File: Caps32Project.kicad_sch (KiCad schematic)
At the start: 37 parts, among them J1 Ph 2.0, J2 Sh 1.0, J4 Sh 2.0, P1 USB_C_Plug_USB2.0, Q1 AO3401A, Q2 MBT3904DW1, SW1 Reset, SW2 Boot, U1 MPU-6050, U2 MAX17048G_T10, U4 MCP73831-2-OT, U5 AP2112K-3.3, U6 ESP32-WROOM-32D

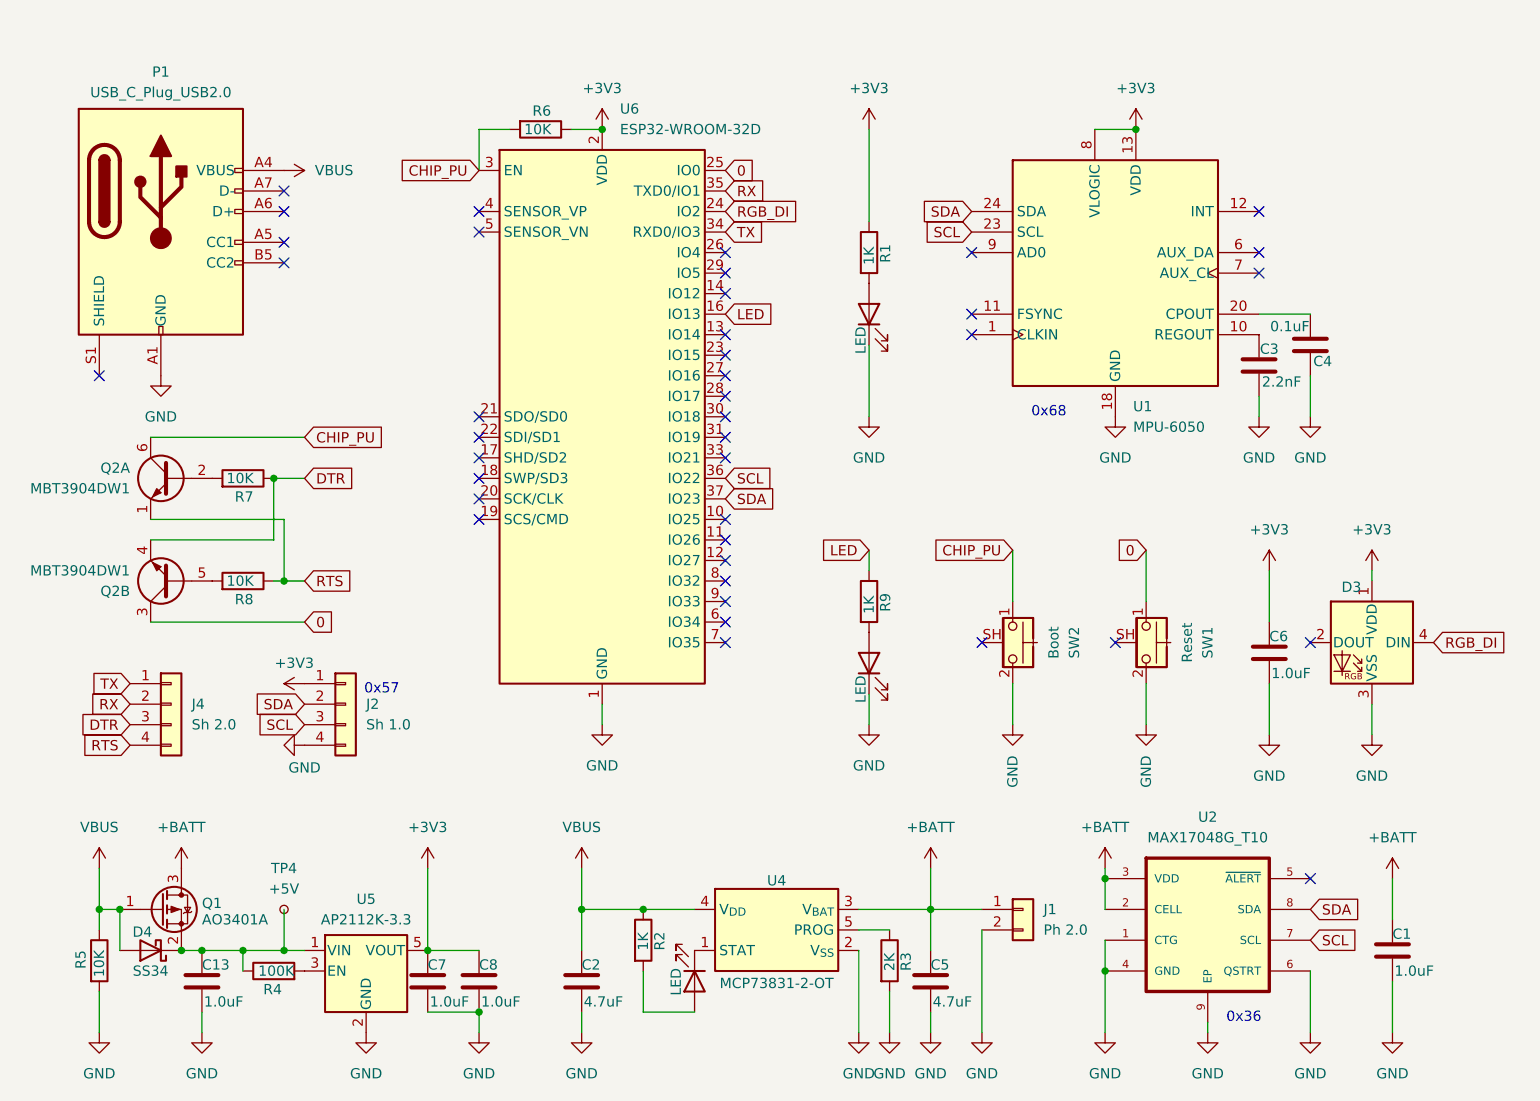
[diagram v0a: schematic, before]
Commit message: Update Board
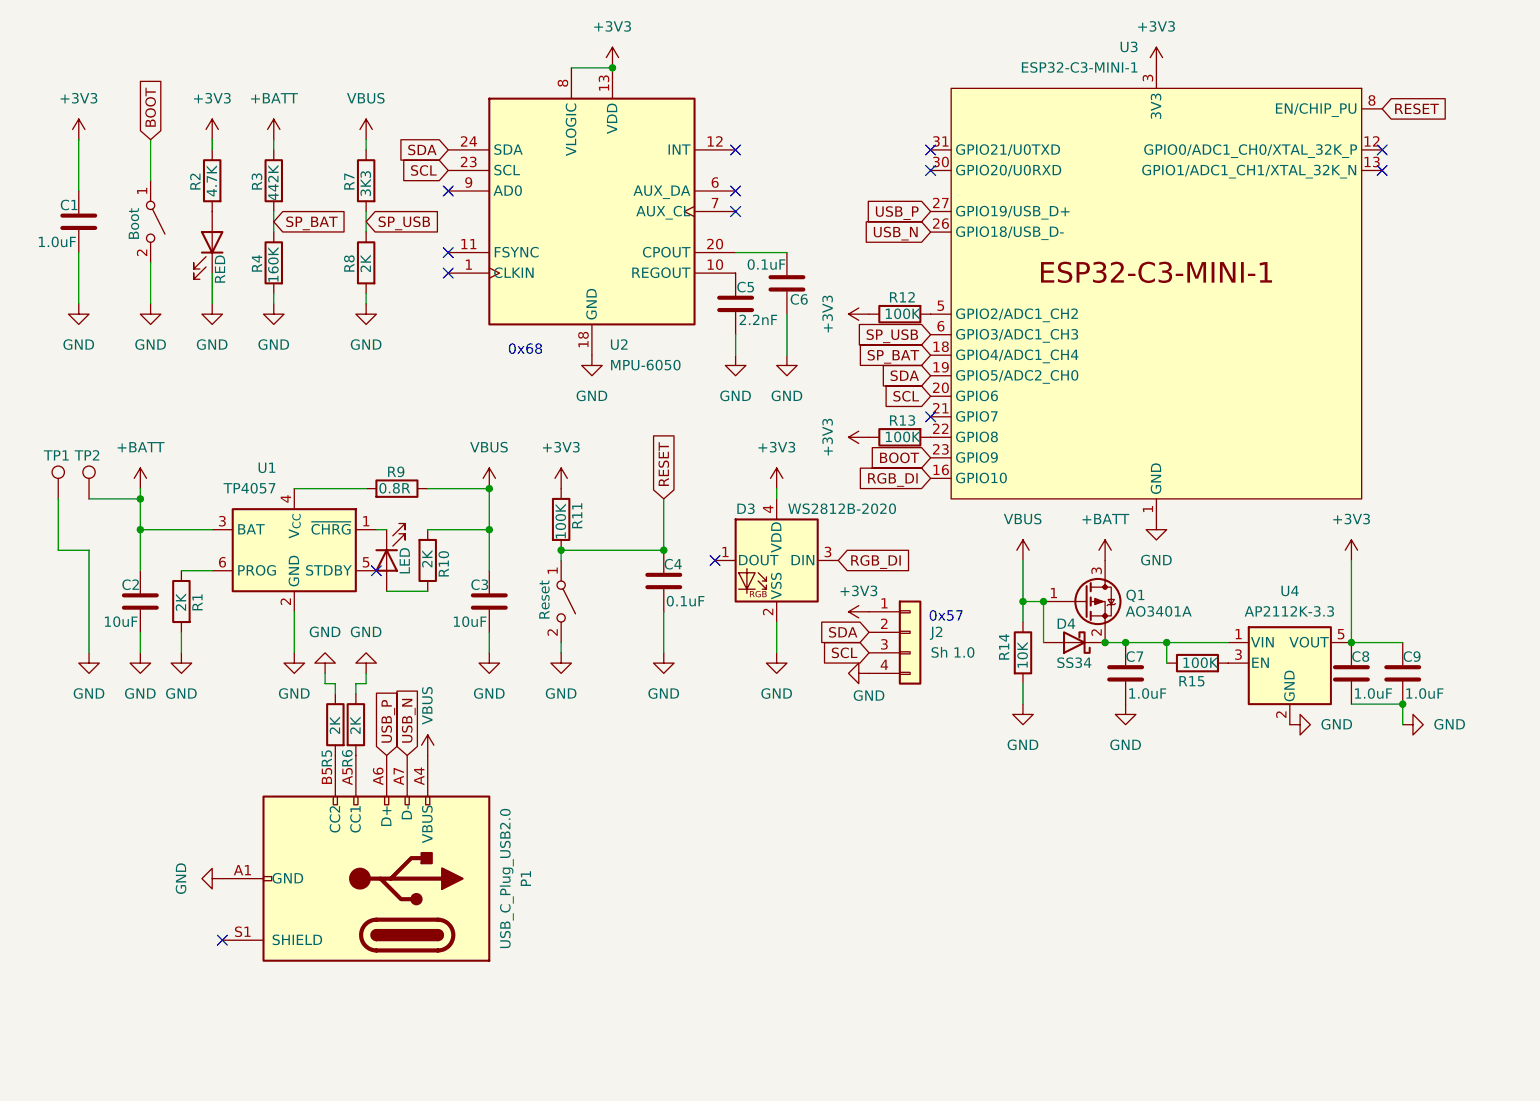
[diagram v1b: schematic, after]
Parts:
- removed C1: 1.0uF, Capacitor_SMD:C_0402_1005Metric_Pad0.74x0.62mm_HandSolder, symbol Device:C
- removed D3: WS2812B, LED_SMD:LED_WS2812B_PLCC4_5.0x5.0mm_P3.2mm, symbol LED:WS2812B
- removed D5: LED, LED_SMD:LED_0402_1005Metric_Pad0.77x0.64mm_HandSolder, symbol Device:LED
- removed J1: Ph 2.0, Connector_JST:JST_PH_S2B-PH-SM4-TB_1x02-1MP_P2.00mm_Horizontal, symbol Connector_Generic:Conn_01x02
- removed J4: Sh 2.0, Connector_JST:JST_SH_SM04B-SRSS-TB_1x04-1MP_P1.00mm_Horizontal, symbol Connector_Generic:Conn_01x04
- removed Q2: MBT3904DW1, Package_TO_SOT_SMD:SOT-363_SC-70-6, symbol Transistor_BJT:MBT3904DW1
- removed SW1: Reset, Button_Switch_SMD:SW_SPST_CK_KMS2xxGP, symbol Switch:CK_KMS2xxGP
- removed SW2: Boot, Button_Switch_SMD:SW_SPST_CK_KMS2xxGP, symbol Switch:CK_KMS2xxGP
- removed TP4: +5V, TestPoint:TestPoint_Pad_D1.0mm, symbol Connector:TestPoint_Small
- removed U1: MPU-6050, Sensor_Motion:InvenSense_QFN-24_4x4mm_P0.5mm, symbol Sensor_Motion:MPU-6050
- removed U2: MAX17048G_T10, Custom:SON50P200X200X80-9N, symbol Custom:MAX17048G_T10
- removed U4: MCP73831-2-OT, Package_TO_SOT_SMD:SOT-23-5, symbol Battery_Management:MCP73831-5-OT
- removed U6: ESP32-WROOM-32D, RF_Module:ESP32-WROOM-32D, symbol RF_Module:ESP32-WROOM-32D
- added C4: 0.1uF, Capacitor_SMD:C_0201_0603Metric, symbol Device:C
- added D3: WS2812B-2020, LED_SMD:LED_WS2812B-2020_PLCC4_2.0x2.0mm, symbol LED:WS2812B-2020
- added R11, R12, R13: 100K, Resistor_SMD:R_0201_0603Metric, symbol Device:R
- added R3: 442K, Resistor_SMD:R_0805_2012Metric, symbol Device:R
- added R4: 160K, Resistor_SMD:R_0805_2012Metric, symbol Device:R
- added R5: 2K, Resistor_SMD:R_0402_1005Metric, symbol Device:R
- added SW1: Boot, Button_Switch_SMD:SW_SPST_CK_KMS2xxGP, symbol Switch:SW_SPST
- added SW2: Reset, Button_Switch_SMD:SW_SPST_CK_KMS2xxGP, symbol Switch:SW_SPST
- added TP1, TP2: TestPoint, TestPoint:TestPoint_Pad_D1.5mm, symbol Connector:TestPoint
- added U1: TP4057, Package_TO_SOT_SMD:TSOT-23-6, symbol Battery_Management:TP4057
- added U2: MPU-6050, Sensor_Motion:InvenSense_QFN-24_4x4mm_P0.5mm_NoMask, symbol Sensor_Motion:MPU-6050
- added U3: ESP32-C3-MINI-1, PCM_Espressif:ESP32-C3-MINI-1, symbol PCM_Espressif:ESP32-C3-MINI-1
- C1: renamed from C6; footprint Capacitor_SMD:C_0402_1005Metric_Pad0.74x0.62mm_HandSolder -> Capacitor_SMD:C_0201_0603Metric
- C2: renamed from C5; value 4.7uF -> 10uF; footprint Capacitor_SMD:C_0402_1005Metric_Pad0.74x0.62mm_HandSolder -> Capacitor_SMD:C_0402_1005Metric
- C3: renamed from C2; value 4.7uF -> 10uF; footprint Capacitor_SMD:C_0402_1005Metric_Pad0.74x0.62mm_HandSolder -> Capacitor_SMD:C_0402_1005Metric
- C5: renamed from C3; footprint Capacitor_SMD:C_0402_1005Metric_Pad0.74x0.62mm_HandSolder -> Capacitor_SMD:C_0603_1608Metric
- C6: renamed from C4; footprint Capacitor_SMD:C_0402_1005Metric_Pad0.74x0.62mm_HandSolder -> Capacitor_SMD:C_0201_0603Metric
- C7: renamed from C13; footprint Capacitor_SMD:C_0402_1005Metric_Pad0.74x0.62mm_HandSolder -> Capacitor_SMD:C_0201_0603Metric
- C8: renamed from C7; footprint Capacitor_SMD:C_0402_1005Metric_Pad0.74x0.62mm_HandSolder -> Capacitor_SMD:C_0201_0603Metric
- C9: renamed from C8; footprint Capacitor_SMD:C_0402_1005Metric_Pad0.74x0.62mm_HandSolder -> Capacitor_SMD:C_0201_0603Metric
- D1: value LED -> RED; footprint LED_SMD:LED_0402_1005Metric_Pad0.77x0.64mm_HandSolder -> LED_SMD:LED_0402_1005Metric
- D2: footprint LED_SMD:LED_0402_1005Metric_Pad0.77x0.64mm_HandSolder -> LED_SMD:LED_0402_1005Metric
- P1: footprint Connector_USB:USB_C_Receptacle_XKB_U262-16XN-4BVC11 -> Connector_USB:USB_C_Receptacle_GCT_USB4105-xx-A_16P_TopMnt_Horizontal
- R1: renamed from R3; footprint Resistor_SMD:R_0402_1005Metric_Pad0.72x0.64mm_HandSolder -> Resistor_SMD:R_0201_0603Metric
- R10: renamed from R2; value 1K -> 2K; footprint Resistor_SMD:R_0402_1005Metric_Pad0.72x0.64mm_HandSolder -> Resistor_SMD:R_0201_0603Metric
- R14: renamed from R5; footprint Resistor_SMD:R_0402_1005Metric_Pad0.72x0.64mm_HandSolder -> Resistor_SMD:R_0201_0603Metric
- R15: renamed from R4; footprint Resistor_SMD:R_0402_1005Metric_Pad0.72x0.64mm_HandSolder -> Resistor_SMD:R_0201_0603Metric
- R2: renamed from R1; value 1K -> 4.7K; footprint Resistor_SMD:R_0402_1005Metric_Pad0.72x0.64mm_HandSolder -> Resistor_SMD:R_0201_0603Metric
- R6: value 10K -> 2K; footprint Resistor_SMD:R_0402_1005Metric_Pad0.72x0.64mm_HandSolder -> Resistor_SMD:R_0402_1005Metric
- R7: value 10K -> 3K3; footprint Resistor_SMD:R_0402_1005Metric_Pad0.72x0.64mm_HandSolder -> Resistor_SMD:R_0201_0603Metric
- R8: value 10K -> 2K; footprint Resistor_SMD:R_0402_1005Metric_Pad0.72x0.64mm_HandSolder -> Resistor_SMD:R_0201_0603Metric
- R9: value 1K -> 0.8R; footprint Resistor_SMD:R_0402_1005Metric_Pad0.72x0.64mm_HandSolder -> Resistor_SMD:R_0201_0603Metric
- renumbered U5 to U4
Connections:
- net CHIP_PU is gone; now on an unnamed net: R6.2
- net DTR is gone; now on net VBUS: R7.1
- net LED is gone; now on net VBUS: R9.1
- net RTS is gone; now on net SP_USB: R8.1
- net +3V3: now also D3.4 (VDD), R11.1, R12.1, R13.1, U2.13 (VDD), U2.8 (VLOGIC), U3.3 (3V3); no longer R6.1
- net +BATT: now also R3.1, TP2.1, U1.3 (BAT)
- net GND: now also R6.1, R8.2, C4.2, D3.2 (VSS), R4.2, R5.1, SW1.2 (B), SW2.2 (B), TP1.1, U1.2 (GND), U2.18 (GND), U3.1 (GND), U3.11 (GND), U3.14 (GND), U3.2 (GND), U3.36 (GND), U3.37 (GND), U3.38 (GND), U3.39 (GND), U3.40 (GND), U3.41 (GND), U3.42 (GND), U3.43 (GND), U3.44 (GND), U3.45 (GND), U3.46 (GND), U3.47 (GND), U3.48 (GND), U3.49 (GND), U3.50 (GND), U3.51 (GND), U3.52 (GND), U3.53 (GND)
- net RGB_DI: now also D3.3 (DIN), U3.16 (GPIO10)
- net SCL: now also U2.23 (SCL), U3.20 (GPIO6)
- net SDA: now also U2.24 (SDA), U3.19 (GPIO5/ADC2_CH0)
- net VBUS: now also R10.2; no longer R10.1
- net at C5.2: now also U2.10 (REGOUT)
- net at C6.1: now also U2.20 (CPOUT)
- net at R1.1: now also U1.6 (PROG)
- net SP_USB: now reaches R7.2
- net SP_USB: now also U3.6 (GPIO3/ADC1_CH3)
- net at D2.1 (K): now also U1.1 (~{CHRG})
- net at D2.2 (A): now also R10.1; no longer R10.2
- net at R9.2: now also U1.4 (V_{CC})
- net USB_P: now reaches P1.A6 (D+)
- net USB_P: now also U3.27 (GPIO19/USB_D+)
- net USB_N: now reaches P1.A7 (D-)
- net USB_N: now also U3.26 (GPIO18/USB_D-)
- net at P1.B5 (CC2): now also R5.2
- new net: R13.2, U3.22 (GPIO8)
- new net: R12.2, U3.5 (GPIO2/ADC1_CH2)
- new net BOOT: SW1.1 (A), U3.23 (GPIO9)
- new net RESET: C4.1, R11.2, SW2.1 (A), U3.8 (EN/CHIP_PU)
- new net SP_BAT: R3.2, R4.1, U3.18 (GPIO4/ADC1_CH4)
- no-connect marks 40 -> 14
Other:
- moved on the sheet: C1, C2, C3, C5, C6, C7, C8, C9, D4, J2, P1, Q1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
